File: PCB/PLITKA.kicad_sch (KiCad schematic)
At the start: 55 parts, among them SW1 MX_SW_HS, SW10 MX_SW_HS, SW11 MX_SW_HS, SW12 MX_SW_HS, SW13 MX_SW_HS, SW14 MX_SW_HS, SW15 MX_SW_HS, SW16 MX_SW_HS, SW17 MX_SW_HS, SW18 RotaryEncoder, SW2 MX_SW_HS, SW3 MX_SW_HS, SW4 MX_SW_HS, SW5 MX_SW_HS, SW6 MX_SW_HS, SW7 MX_SW_HS, SW8 MX_SW_HS, SW9 MX_SW_HS, U1 nice!nano

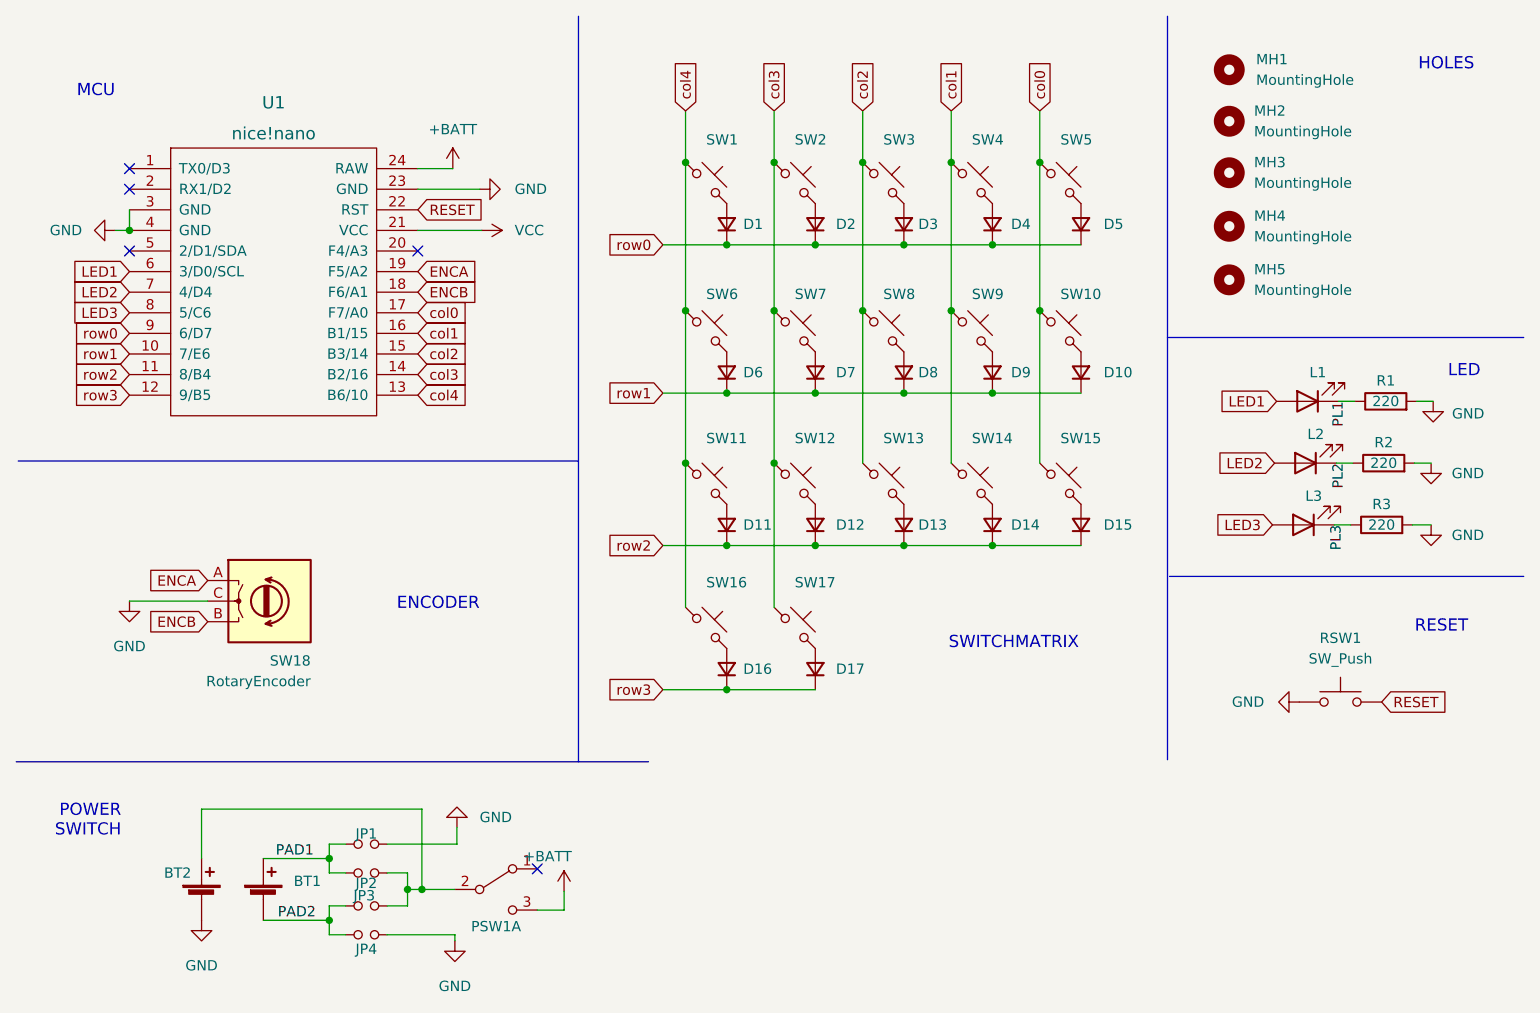
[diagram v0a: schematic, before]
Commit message: KiCad versions update
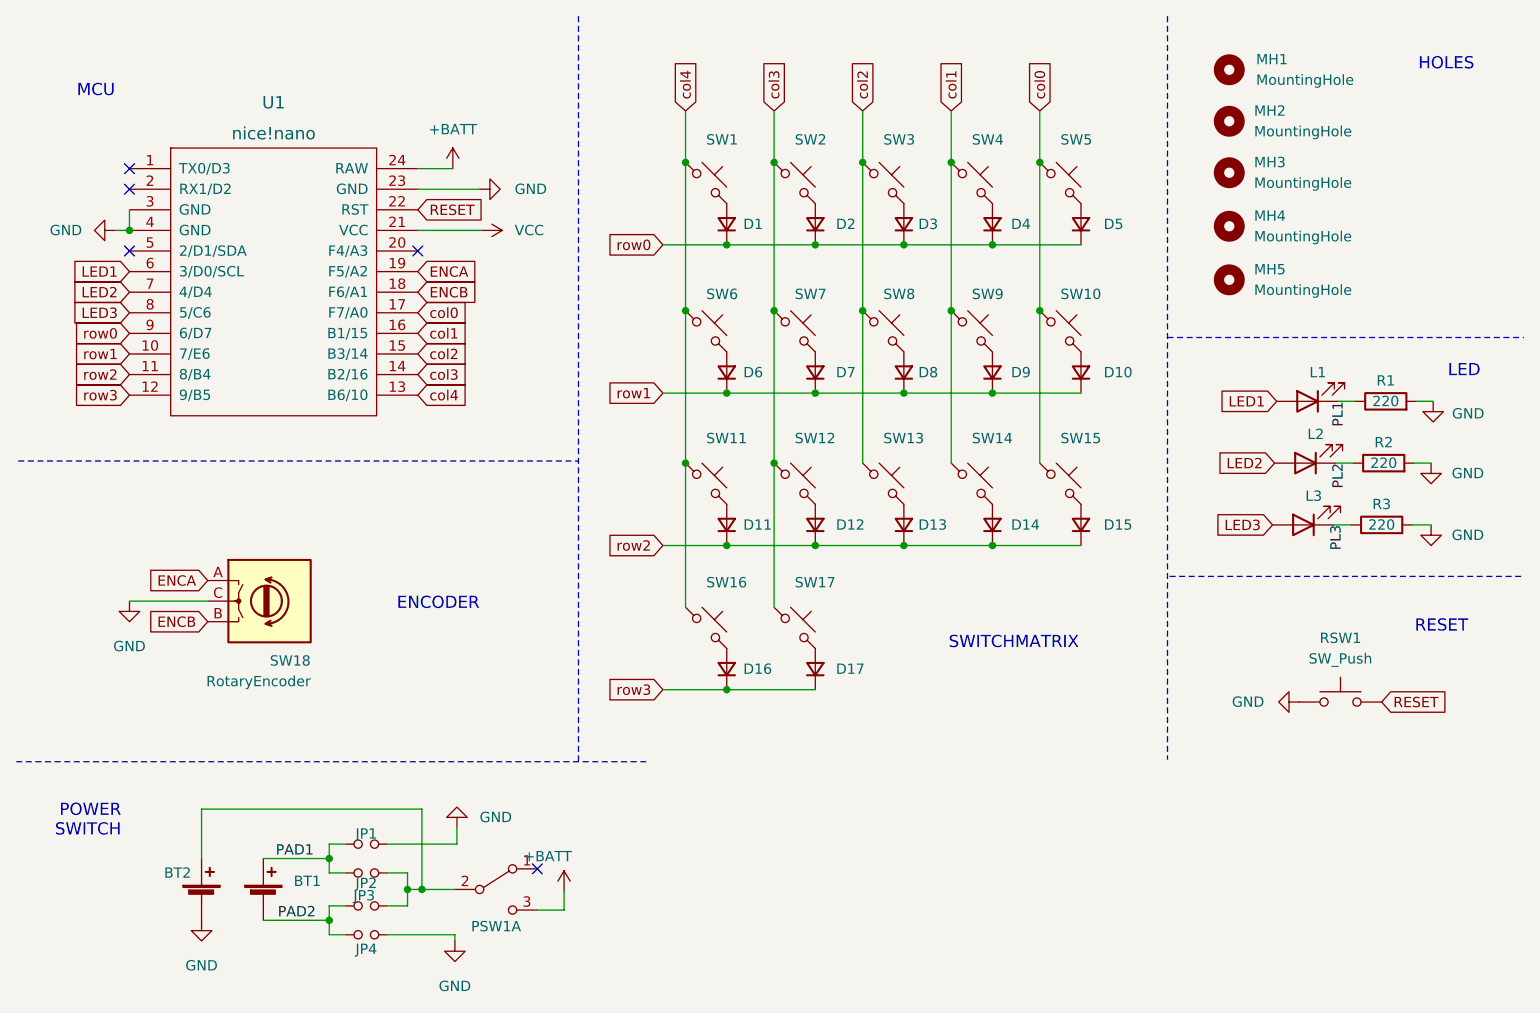
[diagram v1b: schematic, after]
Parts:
- RSW1: footprint (none) -> PLITKA:ResetSW
